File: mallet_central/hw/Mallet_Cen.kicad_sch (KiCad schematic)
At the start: 23 parts, among them J1 Barrel_Jack_Switch_Pin3Ring, J2 Conn_01x04, J3 Conn_01x08, J4 Conn_01x04, U1 MT2492, U2 STM32G030F6Px, U3 LTC4311CSC6#TRPBF

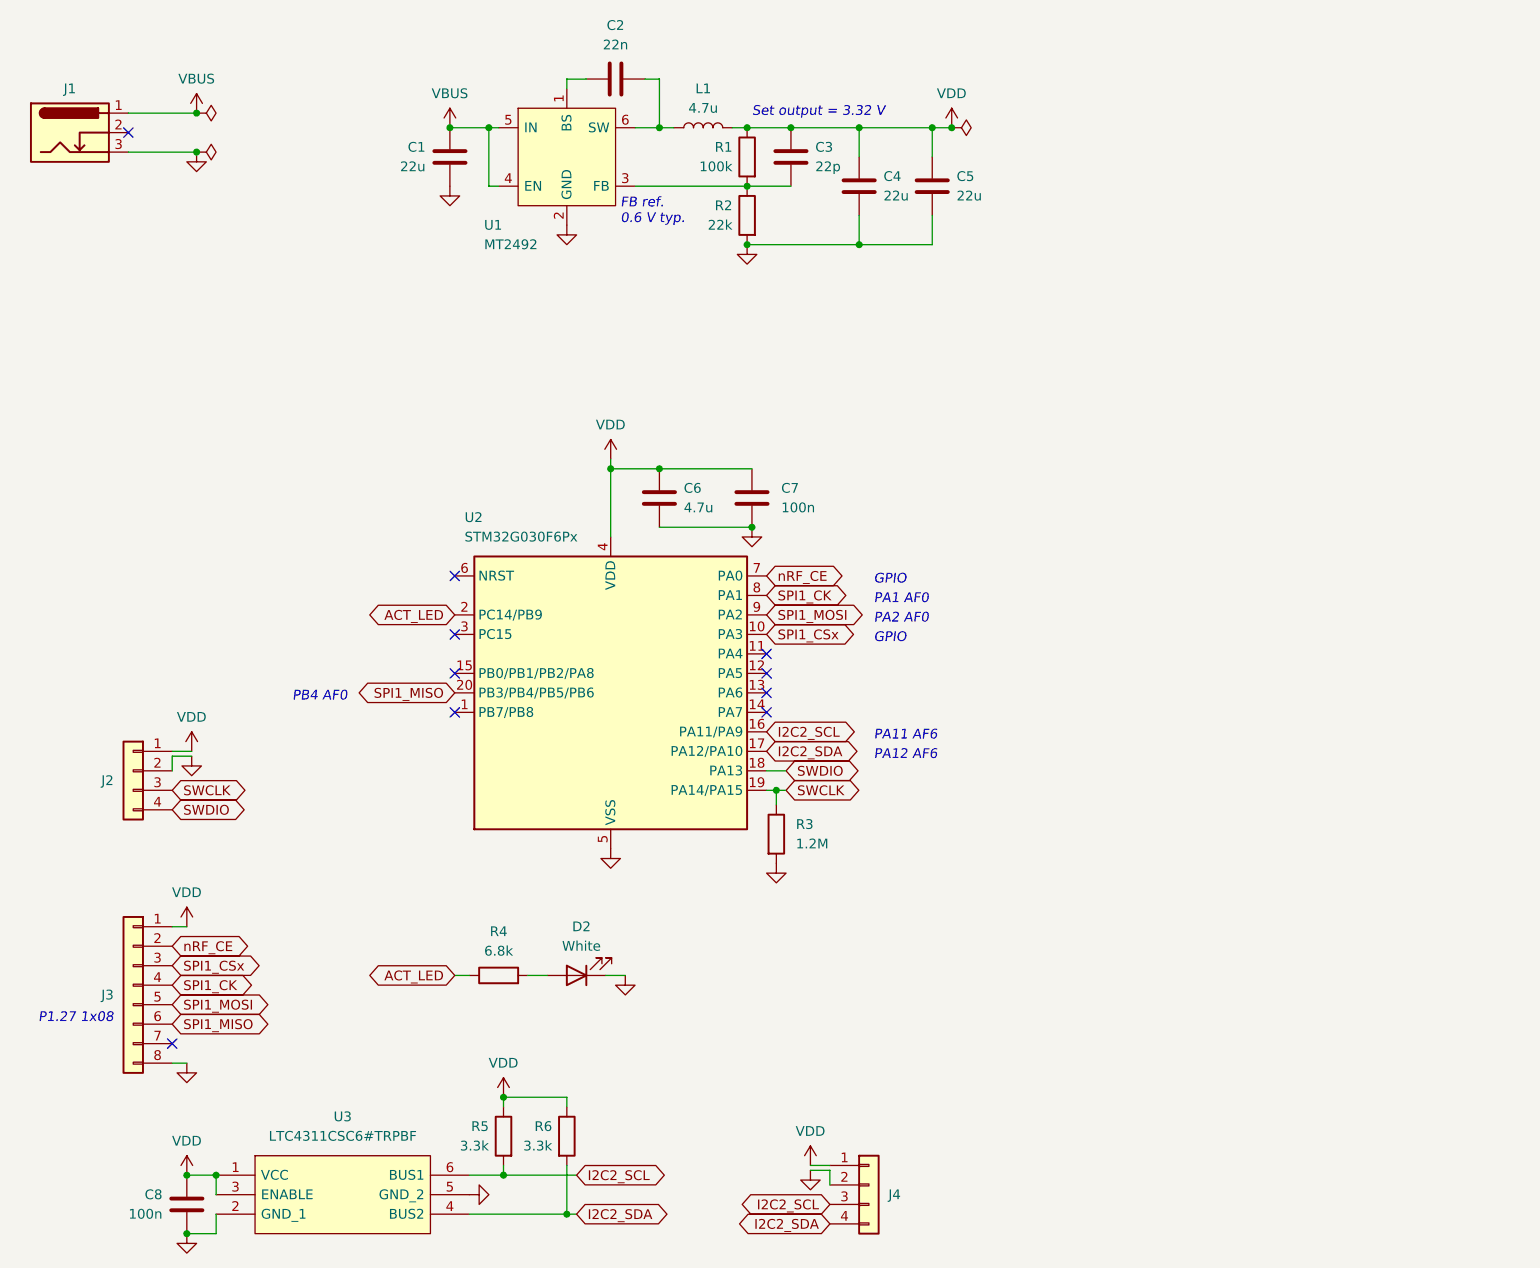
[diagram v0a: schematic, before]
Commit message: Revise central module hardware design
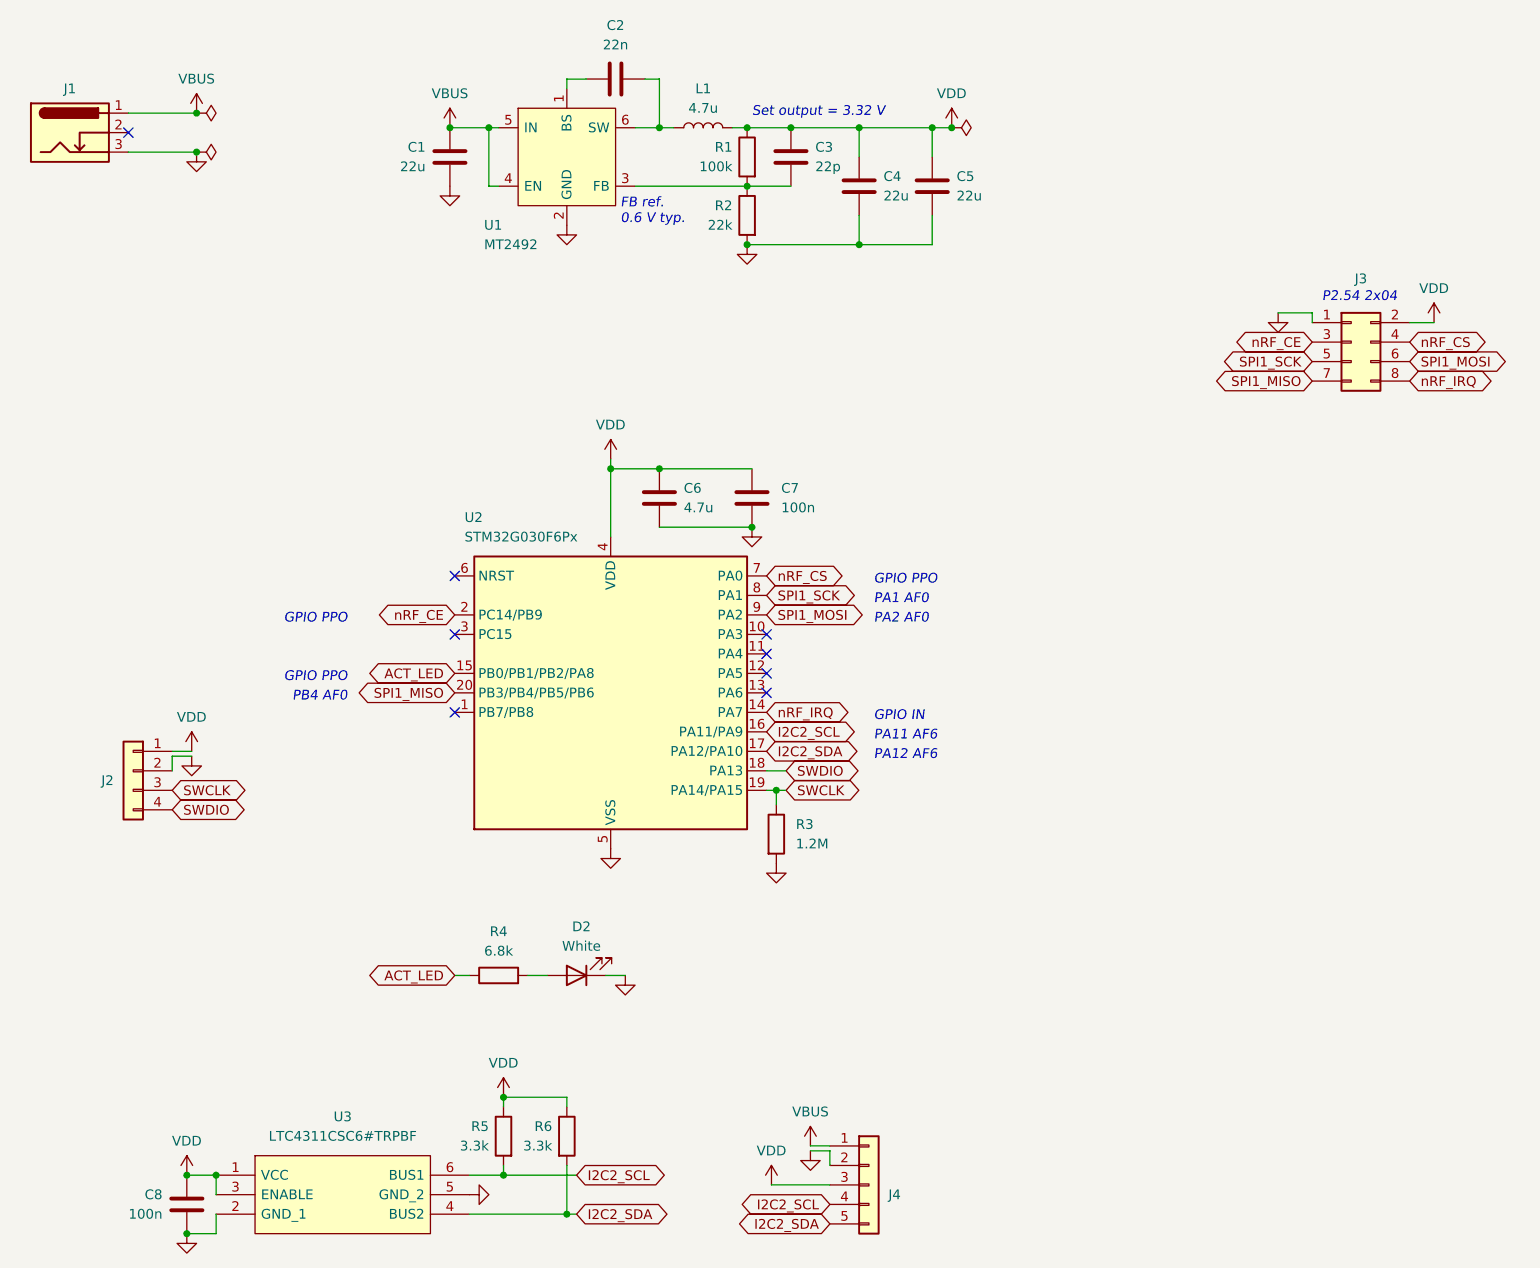
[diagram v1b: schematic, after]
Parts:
- removed J3: Conn_01x08, Mallet_Cen_footprints:SMD_Module_P1.27_1x08, symbol Connector_Generic:Conn_01x08
- added J3: Conn_02x04_Odd_Even, Connector_PinSocket_2.54mm:PinSocket_2x04_P2.54mm_Vertical, symbol Connector_Generic:Conn_02x04_Odd_Even
- J4: value Conn_01x04 -> Conn_01x05; footprint Connector_PinHeader_2.00mm:PinHeader_1x04_P2.00mm_Vertical -> Connector_PinHeader_2.00mm:PinHeader_1x05_P2.00mm_Vertical; symbol Connector_Generic:Conn_01x04 -> Connector_Generic:Conn_01x05
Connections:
- net ACT_LED: now also U2.15 (PB0/PB1/PB2/PA8); no longer U2.2 (PC14/PB9)
- net GND: now also J3.1 (Pin_1)
- net I2C2_SCL: now also J4.4 (Pin_4); no longer J4.3 (Pin_3)
- net I2C2_SDA: now also J4.5 (Pin_5); no longer J4.4 (Pin_4)
- net SPI1_MISO: now also J3.7 (Pin_7)
- net SPI1_MOSI: now also J3.6 (Pin_6)
- net VBUS: now also J4.1 (Pin_1)
- net VDD: now also J4.3 (Pin_3), J3.2 (Pin_2); no longer J4.1 (Pin_1)
- net nRF_CE: now also U2.2 (PC14/PB9), J3.3 (Pin_3); no longer U2.7 (PA0)
- net nRF_IRQ: now reaches U2.14 (PA7)
- net nRF_IRQ: now also J3.8 (Pin_8)
- net SPI1_CK renamed SPI1_SCK
- net SPI1_SCK: now also J3.5 (Pin_5)
- net SPI1_CSx: no longer names the net of U2.10 (PA3)
- new net nRF_CS: J3.4 (Pin_4), U2.7 (PA0)
- no-connect marks 10 -> 8
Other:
- note added: "GPIO IN"
- note added: "GPIO PPO"
- note added: "P2.54 2x04"
- note removed: "GPIO"
- note removed: "P1.27 1x08"
